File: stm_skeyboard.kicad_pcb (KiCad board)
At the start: 2 copper layers, 201 x 75 mm, 84 parts, among them J1 USB4085-GF-A, J3 Conn_01x04_Pin, SW1 SW_Push, SW10 SW_Push, SW11 SW_Push, SW12 SW_Push, SW13 SW_Push, SW14 SW_Push, SW15 SW_Push, SW16 SW_Push, SW17 SW_Push, SW18 SW_Push, SW19 SW_Push, SW2 SW_Push, SW20 SW_Push, SW21 SW_Push, SW22 SW_Push, SW23 SW_Push, SW24 SW_Push, SW25 SW_Push, SW26 SW_Push, SW27 SW_Push, SW28 SW_Push, SW29 SW_Push, SW3 SW_Push, SW30 SW_Push, SW31 SW_Push, SW4 SW_Push, SW5 SW_Push, SW6 SW_Push, SW7 SW_Push, SW8 SW_Push, SW9 SW_Push, U1 TPS7B8133DRVR, U2 STM32L053C8T6

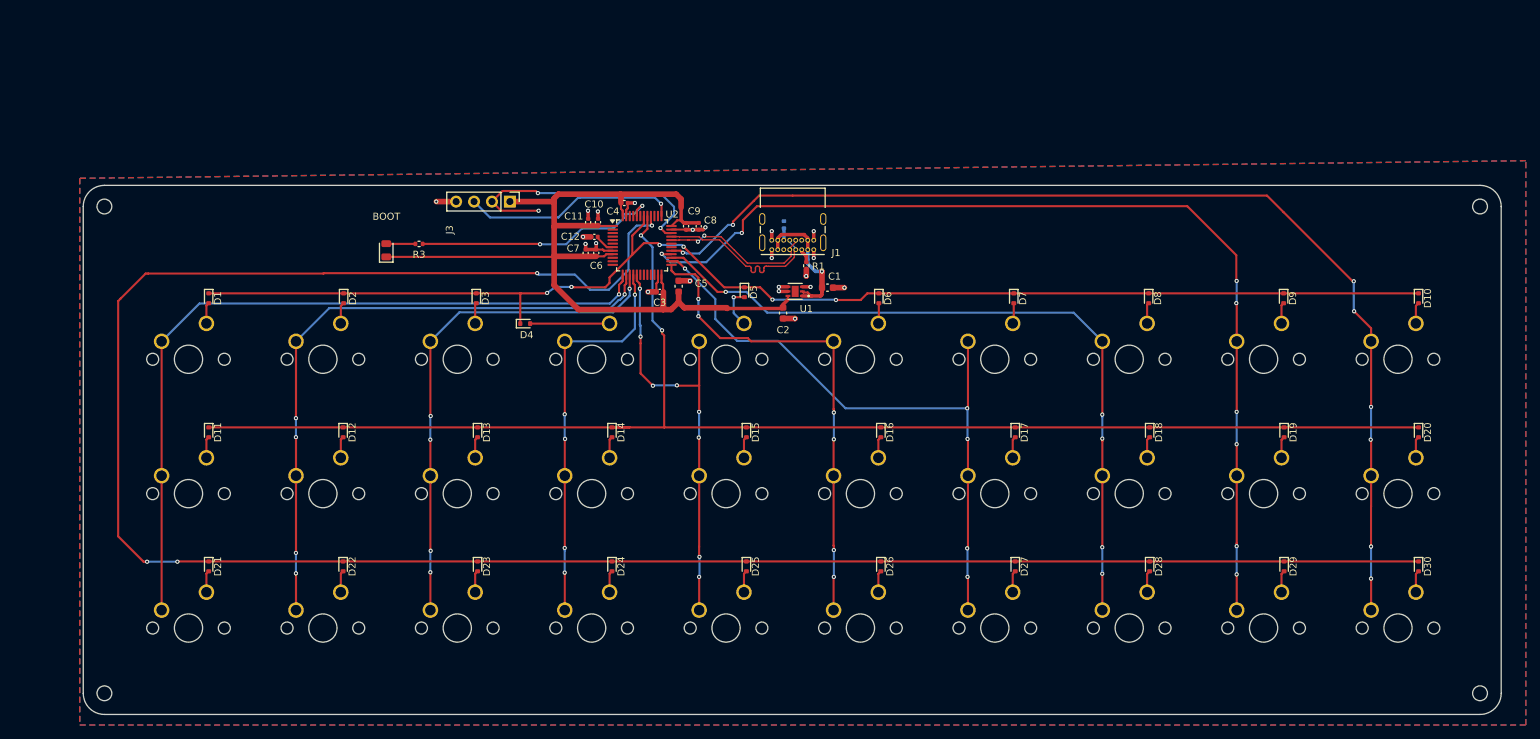
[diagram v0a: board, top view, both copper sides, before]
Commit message: re-done whole pcb
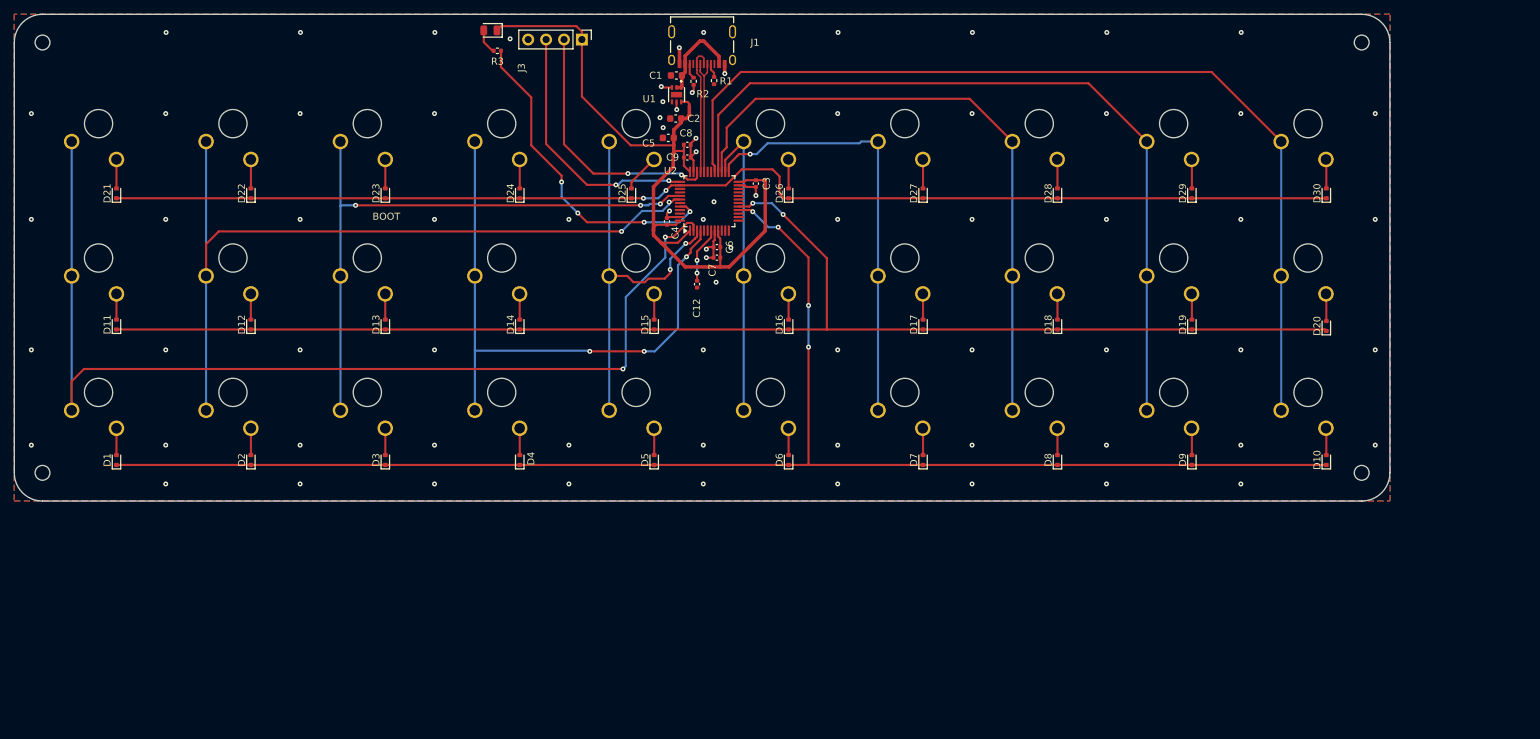
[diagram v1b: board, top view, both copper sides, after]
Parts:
- removed C10: 100n, Capacitor_SMD:C_0402_1005Metric
- removed C11: 1u, Capacitor_SMD:C_0402_1005Metric
- J1: value USB4085-GF-A -> GSB1C411111DS1HR; footprint Connector_USB:USB_C_Receptacle_GCT_USB4085 -> usb_personal:AMPHENOL_GSB1C411111DS1HR
- R2: moved to F.Cu
- SW1, SW10, SW11, SW12, SW13, SW14, SW15, SW16, SW17, SW18, SW19, SW2, SW20, SW21, SW22, SW23, SW24, SW25, SW26, SW27, SW28, SW29, SW3, SW30, SW4, SW5, SW6, SW7, SW8, SW9: footprint my_switch:SW_Cherry_MX_1.00u_PCB -> my_switch:SW_Cherry_MX_1.00u_PCB_no_support_stems; moved to B.Cu
- moved H4 206.2 mm to (57.2, 124.2)
- moved H3 180.9 mm to (244.2, 124.2)
- moved SW21 62.7 mm to (67.7, 79.8)
- moved SW22 62.7 mm to (86.8, 79.8)
- moved SW23 62.7 mm to (105.8, 79.8)
- moved SW24 62.7 mm to (124.9, 79.8)
- moved SW25 62.7 mm to (143.9, 79.8)
- moved SW26 62.7 mm to (163.0, 79.8)
- moved SW27 62.7 mm to (182.0, 79.8)
- moved SW28 62.7 mm to (201.1, 79.8)
- moved SW29 62.7 mm to (220.1, 79.8)
- moved SW30 62.7 mm to (239.2, 79.8)
- moved D25 55.3 mm to (140.7, 84.6), turned to 90 degrees
- moved D21 54.5 mm to (67.7, 84.6), turned to 90 degrees
- moved D22 54.5 mm to (86.8, 84.6), turned to 90 degrees
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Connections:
- U2 pad 13: /matrix/COL0 -> unconnected-(U2-PA3-Pad13)
- U2 pad 14: /matrix/COL1 -> unconnected-(U2-PA4-Pad14)
- U2 pad 15: /matrix/COL2 -> unconnected-(U2-PA5-Pad15)
- U2 pad 16: /matrix/COL3 -> /matrix/ROW0
- U2 pad 17: /matrix/COL4 -> /matrix/ROW1
- U2 pad 2: unconnected-(U2-PC13-Pad2) -> /matrix/COL0
- U2 pad 25: /matrix/COL5 -> /matrix/COL6
- U2 pad 26: /matrix/COL6 -> /matrix/COL5
- U2 pad 3: unconnected-(U2-PC14-Pad3) -> /matrix/COL4
- U2 pad 38: unconnected-(U2-PA15-Pad38) -> /matrix/ROW2
- U2 pad 4: unconnected-(U2-PC15-Pad4) -> /matrix/COL3
- U2 pad 40: /matrix/ROW2 -> unconnected-(U2-PB4-Pad40)
- U2 pad 41: /matrix/ROW1 -> /matrix/COL2
- U2 pad 42: /matrix/ROW0 -> /matrix/COL1
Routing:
- net /matrix/ROW2: track 305.7 -> 176.4 mm, vias 4 -> 2
- net /matrix/COL0: track 108.7 -> 148.0 mm, vias 1 -> 2
- net /matrix/COL6: track 90.5 -> 61.6 mm, vias 5 -> 1
- net /matrix/COL8: track 140.9 -> 112.2 mm, vias 8 -> 0
- net /matrix/COL3: track 56.6 -> 83.5 mm, vias 5 -> 3
- net /matrix/COL5: track 69.3 -> 43.5 mm, vias 6 -> 0
- net /matrix/ROW0: track 189.1 -> 213.6 mm, vias 6 -> 4
- net /matrix/COL1: track 90.4 -> 112.6 mm, vias 5 -> 2
- net +3.3V: track 131.7 -> 111.6 mm
- net /matrix/COL9: track 153.3 -> 134.7 mm, vias 8 -> 0
- net /matrix/COL7: track 104.1 -> 89.4 mm, vias 5 -> 0
- net /matrix/COL2: track 72.1 -> 86.8 mm, vias 5 -> 3
- net GND: track 38.0 -> 26.8 mm, vias 21 -> 76
- net /mcu/BOOT0: track 35.6 -> 46.4 mm, vias 2 -> 4
- net /matrix/ROW1: track 205.7 -> 197.6 mm
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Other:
- board size 201 x 75 mm -> 195 x 69 mm
